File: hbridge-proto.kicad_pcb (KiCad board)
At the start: 2 copper layers, 125 x 72 mm, 30 parts, among them IC1 LM5106, IC2 LM5106, J1 Screw_Terminal_1x03, J2 Screw_Terminal_1x02, J3 Screw_Terminal_1x02, J4 Screw_Terminal_1x02, Q1 TO-220-DUAL, Q2 TO-220-DUAL, Q3 TO-220-DUAL, Q4 TO-220-DUAL

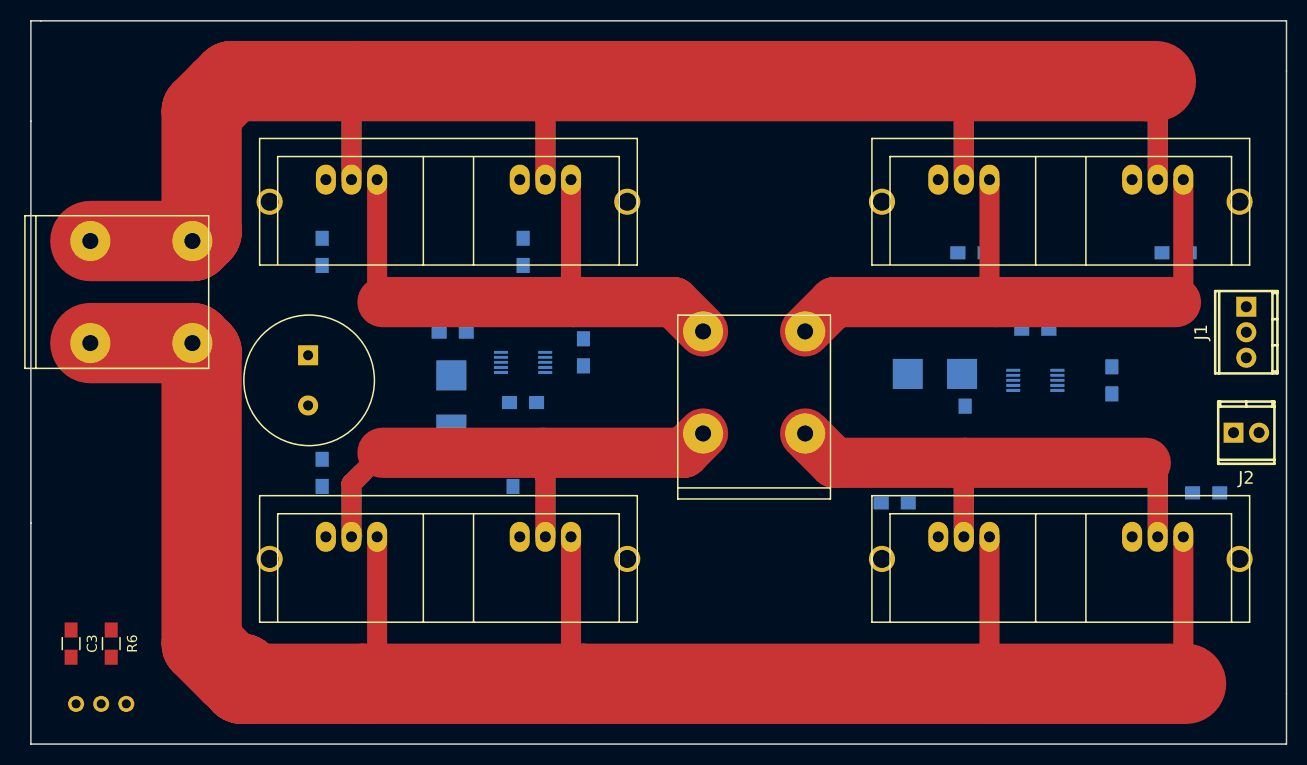
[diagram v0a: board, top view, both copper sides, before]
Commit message: first draft complete
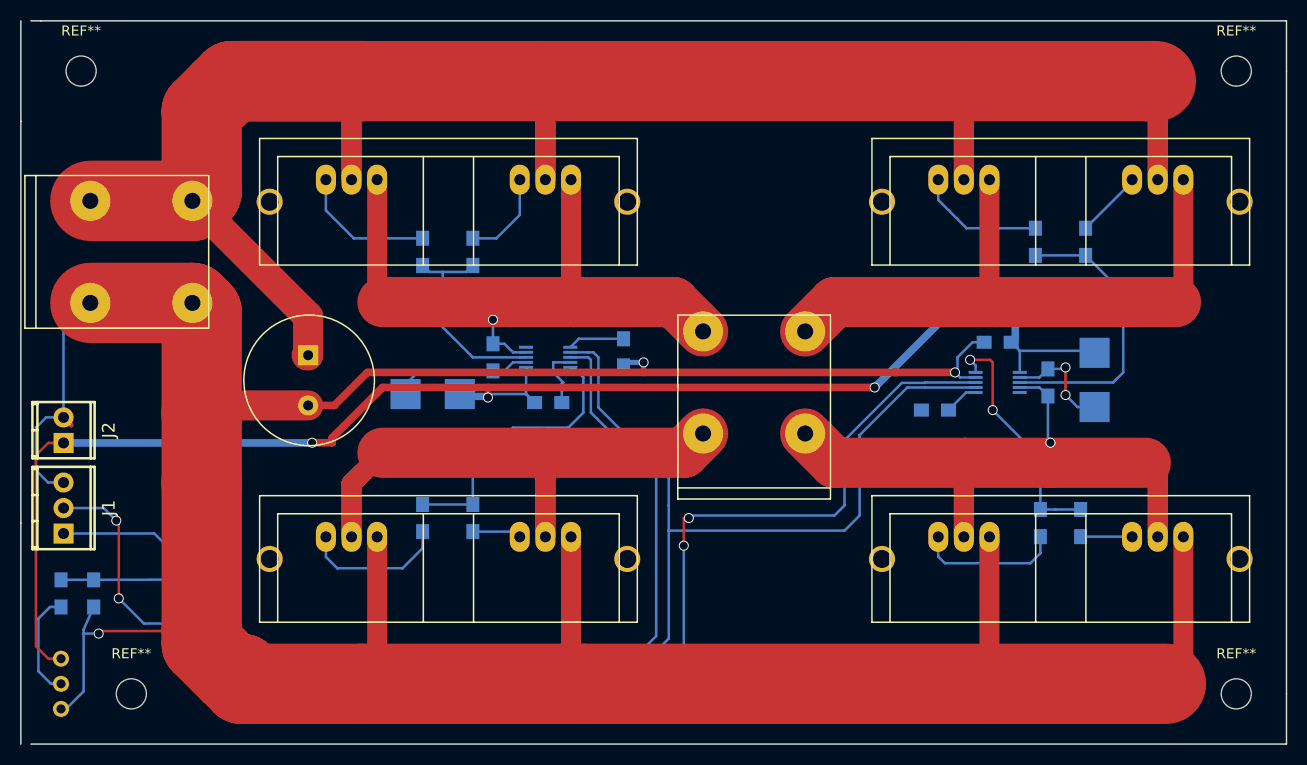
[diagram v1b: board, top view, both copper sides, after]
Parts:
- added REF**: MountingHole_3mm, Mounting_Holes:MountingHole_3mm, F.Cu at (79.0, 67.0)
- added REF**: MountingHole_3mm, Mounting_Holes:MountingHole_3mm, F.Cu at (84.0, 129.0)
- added REF**: MountingHole_3mm, Mounting_Holes:MountingHole_3mm, F.Cu at (194.0, 129.0)
- added REF**: MountingHole_3mm, Mounting_Holes:MountingHole_3mm, F.Cu at (194.0, 67.0)
- C3, R6: moved to B.Cu
- moved J1 119.0 mm to (77.2, 110.5), turned to 270 degrees
- moved J2 117.8 mm to (77.2, 102.8), turned to 270 degrees
- moved R7 29.5 mm to (174.0, 84.0), turned to 270 degrees
- moved R10 28.5 mm to (178.5, 112.0), turned to 90 degrees
- moved R9 27.8 mm to (174.5, 112.0), turned to 90 degrees
- moved R8 27.7 mm to (179.0, 84.0), turned to 270 degrees
- moved R11 17.9 mm to (164.0, 100.8), turned to 0 degrees
- moved D2 14.0 mm to (177.8, 97.8), turned to 270 degrees
- moved R4 11.0 mm to (113.0, 111.5)
- moved R2 10.0 mm to (113.0, 85.0)
- moved C5 8.31 mm to (175.2, 98.0), turned to 90 degrees
- moved R6 7.07 mm to (77.0, 119.0)
- moved R5 6.02 mm to (118.0, 111.5)
- moved C3 5.48 mm to (80.2, 119.0)
- moved D1 5.00 mm to (114.0, 97.0), turned to 180 degrees
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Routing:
- net +12V: track 0.00 -> 154.9 mm, vias 0 -> 3
- net /DRV_EN: track 0.00 -> 144.0 mm
- net GND: track 200.7 -> 344.0 mm, vias 0 -> 3
- net /DRV_2_IN: track 0.00 -> 127.2 mm, vias 0 -> 4
- net /DRV_1_IN: track 0.00 -> 101.2 mm
- net Net-(IC2-Pad3): track 0.00 -> 28.9 mm
- net +24V: track 187.1 -> 215.4 mm
- net Net-(IC1-Pad10): track 0.00 -> 27.1 mm
- net Net-(IC2-Pad10): track 0.00 -> 24.4 mm, vias 0 -> 2
- net Net-(IC1-Pad3): track 0.00 -> 20.6 mm
- net Net-(Q2-Pad1): track 0.00 -> 14.6 mm
- net Net-(Q3-Pad1): track 0.00 -> 14.5 mm
- net Net-(Q1-Pad1): track 0.00 -> 14.4 mm
- net Net-(C2-Pad2): track 0.00 -> 13.9 mm
- net /MOTOR-: track 127.5 -> 140.9 mm, vias 2 -> 3
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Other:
- board size 125 x 72 mm -> 126 x 72 mm
- net class Default: clearance 0.254 -> 0.2
- rule trace_clearance: 0.254 -> 0.2
- rule trace_min: 0.254 -> 0.2032
